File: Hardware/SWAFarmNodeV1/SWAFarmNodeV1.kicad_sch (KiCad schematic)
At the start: 181 parts, among them J1 M12_5P_A_Coded_PowerIn, Q1 IPD50N06S4L-16, U1 TPS26600PWP, U2 TPS54561, U3 TPS563201

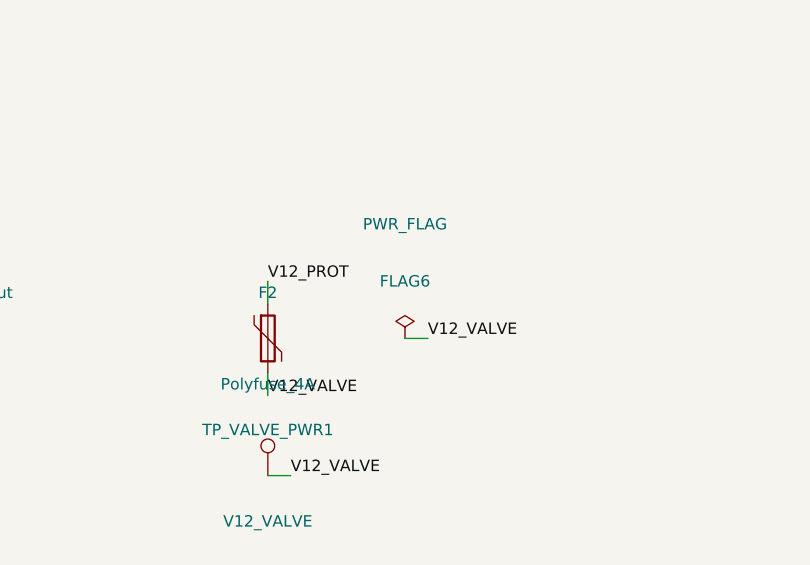
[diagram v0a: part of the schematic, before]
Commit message: updated
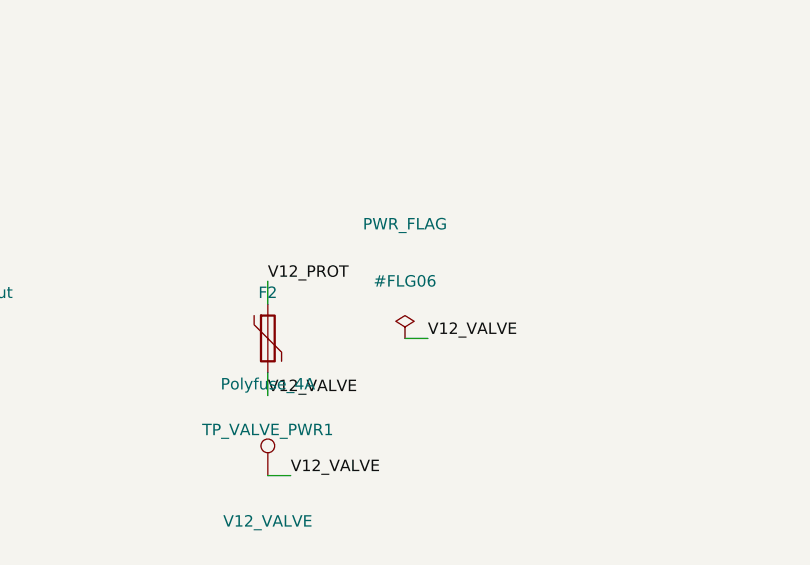
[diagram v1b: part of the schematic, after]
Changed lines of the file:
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@@
 (symbol (lib_id "power:PWR_FLAG") (at 190.5 59.69 0) (unit 1)
 (exclude_from_sim no) (in_bom yes) (on_board yes) (dnp no)
-	(property "Reference" "FLAG6" (at 190.5 53.339999999999996 0)
+	(property "Reference" "#FLG06" (at 190.5 53.339999999999996 0)
 		(effects (font (size 1.27 1.27)))
 	)
@@
 (project "SWAFarmNodeV1"
 (path "/7f190bf9-c800-4055-b329-7f500a7a2cbd"
-(reference "FLAG6")
+(reference "#FLG06")
 (unit 1)
 )
